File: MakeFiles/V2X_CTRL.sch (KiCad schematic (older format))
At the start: 22 parts, among them Q15 2N7000, U18 74HC595, U20 ATXMEGA128A4U-AU, X3 32.768K

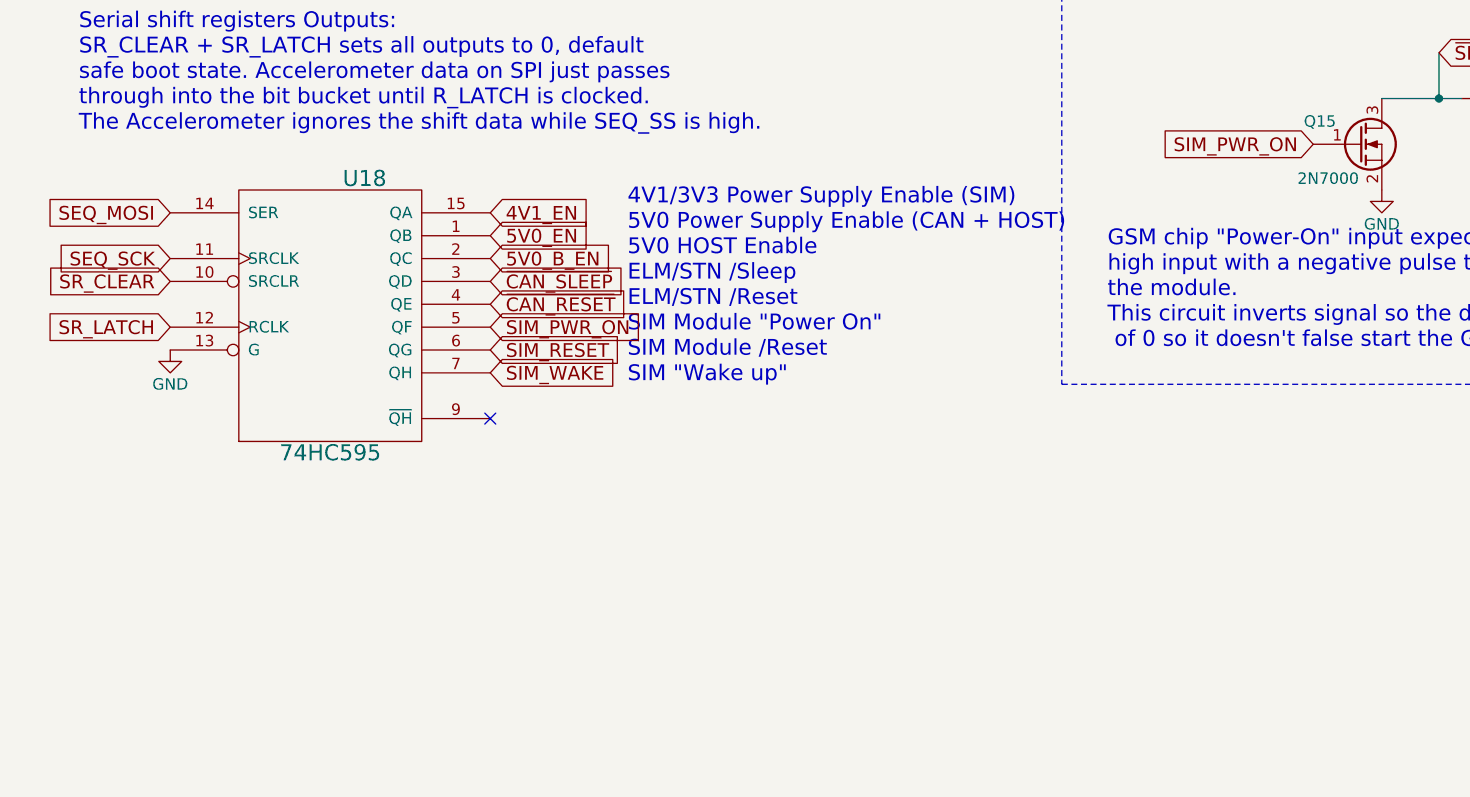
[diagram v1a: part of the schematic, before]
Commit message: Changes for documentation
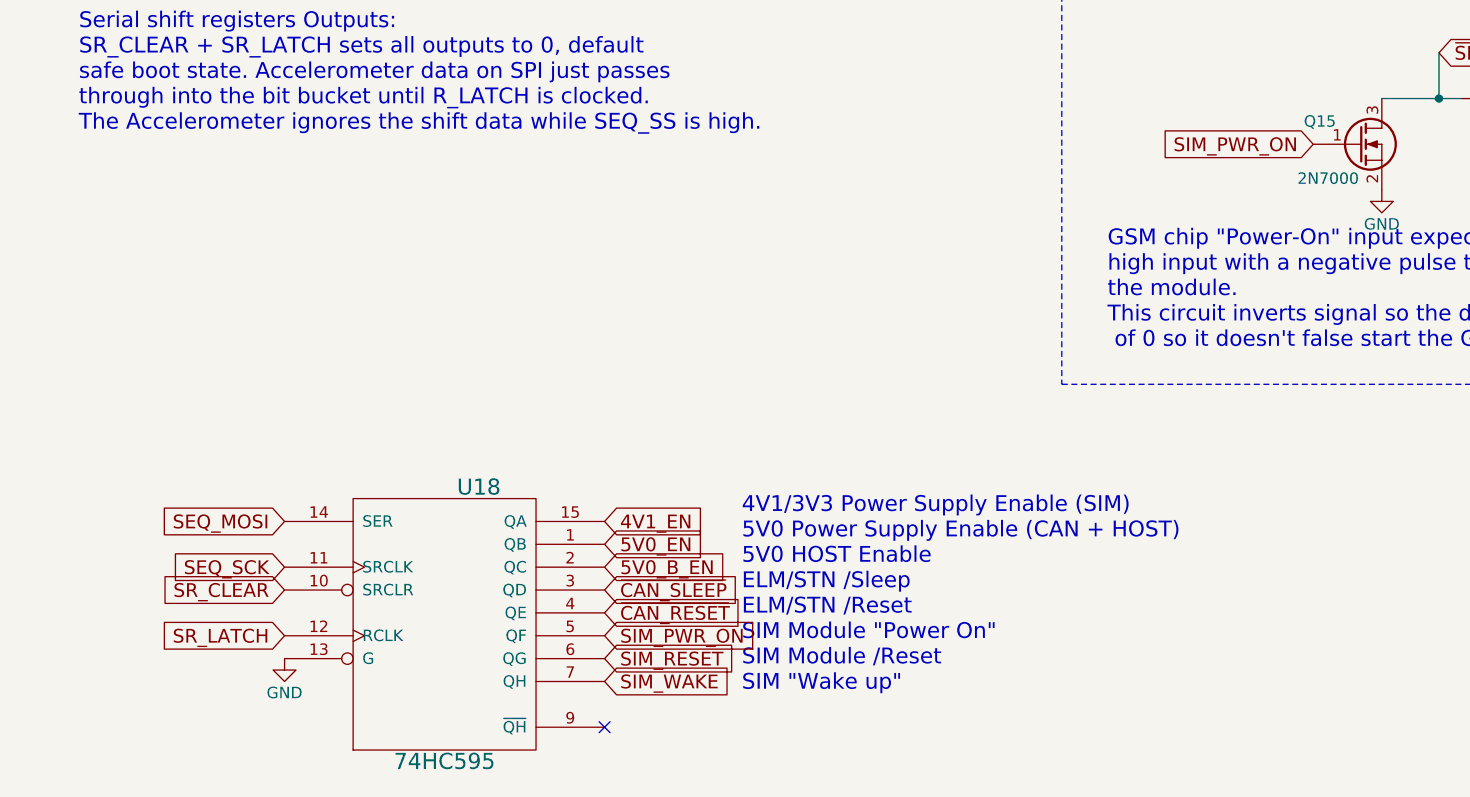
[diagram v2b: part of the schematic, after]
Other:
- moved on the sheet: U18
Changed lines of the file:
@@
 LIBS:xilinx
 LIBS:Zilog
+LIBS:CUSTOM_KICAD_PART
 LIBS:V2X-cache
 EELAYER 25 0
@@
 Text GLabel 6650 4450 2    60   Input ~ 0
 ~SIM_PWR_ON
-Text GLabel 2500 5750 2    60   Input ~ 0
+Text GLabel 3000 7100 2    60   Input ~ 0
 SIM_RESET
 Text GLabel 3350 3400 0    60   Input ~ 0
@@
 Text GLabel 3350 3200 0    60   Input ~ 0
 GPS_EN
-Text GLabel 2500 5150 2    60   Input ~ 0
+Text GLabel 3000 6500 2    60   Input ~ 0
 4V1_EN
-Text GLabel 2500 5250 2    60   Input ~ 0
+Text GLabel 3000 6600 2    60   Input ~ 0
 5V0_EN
 Text GLabel 3350 3000 0    60   Input ~ 0
 SIM_TXD
-Text GLabel 2500 5450 2    60   Input ~ 0
+Text GLabel 3000 6800 2    60   Input ~ 0
 ~CAN_SLEEP
-Text GLabel 2500 5550 2    60   Input ~ 0
+Text GLabel 3000 6900 2    60   Input ~ 0
 ~CAN_RESET
 Text Notes 6050 3600 0    69   ~ 0
@@
 Text Notes 8700 3000 0    60   ~ 0
 PDI (a-wire) Programing port
-Text Notes 3100 5900 0    69   ~ 0
+Text Notes 3600 7250 0    69   ~ 0
 4V1/3V3 Power Supply Enable (SIM)\n5V0 Power Supply Enable (CAN + HOST)\n5V0 HOST Enable \nELM/STN /Sleep\nELM/STN /Reset\nSIM Module "Power On"\nSIM Module /Reset\nSIM "Wake up"
 Text Notes 9700 3250 0    69   ~ 0
@@
 L 74HC595 U18
 U 1 1 55FA3B36
-P 1800 5600
-F 0 "U18" H 1950 6200 70  0000 C CNN
-F 1 "74HC595" H 1800 5000 70  0000 C CNN
-F 2 "Housings_SOIC:SOIC-16_3.9x9.9mm_Pitch1.27mm" H 1800 5600 60  0001 C CNN
-F 3 "http://www.mouser.com/ds/2/302/74HC_HCT595_Q100-269352.pdf" H 1800 5600 60  0001 C CNN
-F 4 "771-74HC595D-Q100" H 1800 5600 60  0001 C CNN "Mouse PN"
-	1    1800 5600
-	1    0    0    -1
-$EndComp
-Text GLabel 2500 5350 2    60   Input ~ 0
+P 2300 6950
+F 0 "U18" H 2450 7550 70  0000 C CNN
+F 1 "74HC595" H 2300 6350 70  0000 C CNN
+F 2 "Housings_SOIC:SOIC-16_3.9x9.9mm_Pitch1.27mm" H 2300 6950 60  0001 C CNN
+F 3 "http://www.mouser.com/ds/2/302/74HC_HCT595_Q100-269352.pdf" H 2300 6950 60  0001 C CNN
+F 4 "771-74HC595D-Q100" H 2300 6950 60  0001 C CNN "Mouse PN"
+	1    2300 6950
+	1    0    0    -1
+$EndComp
+Text GLabel 3000 6700 2    60   Input ~ 0
 5V0_B_EN
 $Comp
 L GND #PWR092
 U 1 1 55FA434A
-P 1100 5750
-F 0 "#PWR092" H 1100 5500 50  0001 C CNN
-F 1 "GND" H 1100 5600 50  0000 C CNN
-F 2 "" H 1100 5750 60  0000 C CNN
-F 3 "" H 1100 5750 60  0000 C CNN
-	1    1100 5750
+P 1600 7100
+F 0 "#PWR092" H 1600 6850 50  0001 C CNN
+F 1 "GND" H 1600 6950 50  0000 C CNN
+F 2 "" H 1600 7100 60  0000 C CNN
+F 3 "" H 1600 7100 60  0000 C CNN
+	1    1600 7100
 	1    0    0    -1
 $EndComp
@@
 Text GLabel 6100 4850 0    60   Input ~ 0
 SIM_PWR_ON
-Text GLabel 2500 5650 2    60   Input ~ 0
+Text GLabel 3000 7000 2    60   Input ~ 0
 SIM_PWR_ON
 Connection ~ 6650 4650
@@
 Text GLabel 7050 4650 2    60   Input ~ 0
 3V3
-Text GLabel 1100 5150 0    60   Input ~ 0
+Text GLabel 1600 6500 0    60   Input ~ 0
 SEQ_MOSI
-Text GLabel 1100 5650 0    60   Input ~ 0
+Text GLabel 1600 7000 0    60   Input ~ 0
 SR_LATCH
-Text GLabel 1100 5450 0    60   Input ~ 0
+Text GLabel 1600 6800 0    60   Input ~ 0
 SR_CLEAR
-Text GLabel 1100 5350 0    60   Input ~ 0
+Text GLabel 1600 6700 0    60   Input ~ 0
 SEQ_SCK
 Wire Notes Line
@@
 Text GLabel 5150 3100 2    60   Input ~ 0
 CAN_RXD
-Text GLabel 2500 5850 2    60   Input ~ 0
+Text GLabel 3000 7200 2    60   Input ~ 0
 SIM_WAKE
 NoConn ~ 9450 3550
@@
 Text GLabel 10650 4900 1    60   Input ~ 0
 4V1
-NoConn ~ 2500 6050
+NoConn ~ 3000 7400
 NoConn ~ 5150 2350
 NoConn ~ 5150 2550

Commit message: Part numer updates
for error or out of stock
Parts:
- C46: Mouse PN 603-CC603KRX7R7BB105 -> 81-GRM188R71C105KA2J
- U20: Mouse PN 556-ATXMEGA16A4U-AU -> 556-ATXMEGA128A4U-AU
- X3: Mouser 628-SC32P-125PF20PPM -> 815-S07AIG-32.76891T
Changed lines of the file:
@@
 SEQ_LED2
 $Comp
-L GND #PWR090
+L GND #PWR93
 U 1 1 55F86E9C
 P 4100 3900
-F 0 "#PWR090" H 4100 3650 50  0001 C CNN
+F 0 "#PWR93" H 4100 3650 50  0001 C CNN
 F 1 "GND" H 4100 3750 50  0000 C CNN
 F 2 "" H 4100 3900 60  0000 C CNN
@@
 PDI
 $Comp
-L GND #PWR091
+L GND #PWR102
 U 1 1 55F86EF0
 P 10000 3650
-F 0 "#PWR091" H 10000 3400 50  0001 C CNN
+F 0 "#PWR102" H 10000 3400 50  0001 C CNN
 F 1 "GND" H 10000 3500 50  0000 C CNN
 F 2 "" H 10000 3650 60  0000 C CNN
@@
 5V0_B_EN
 $Comp
-L GND #PWR092
+L GND #PWR90
 U 1 1 55FA434A
 P 1600 7100
-F 0 "#PWR092" H 1600 6850 50  0001 C CNN
+F 0 "#PWR90" H 1600 6850 50  0001 C CNN
 F 1 "GND" H 1600 6950 50  0000 C CNN
 F 2 "" H 1600 7100 60  0000 C CNN
@@
 $EndComp
 $Comp
-L GND #PWR093
+L GND #PWR94
 U 1 1 55FE1020
 P 6400 5050
-F 0 "#PWR093" H 6400 4800 50  0001 C CNN
+F 0 "#PWR94" H 6400 4800 50  0001 C CNN
 F 1 "GND" H 6400 4900 50  0000 C CNN
 F 2 "" H 6400 5050 60  0000 C CNN
@@
 Connection ~ 10550 750
 $Comp
-L GND #PWR094
+L GND #PWR103
 U 1 1 56006FBB
 P 10550 1100
-F 0 "#PWR094" H 10550 850 50  0001 C CNN
+F 0 "#PWR103" H 10550 850 50  0001 C CNN
 F 1 "GND" H 10550 950 50  0000 C CNN
 F 2 "" H 10550 1100 60  0000 C CNN
@@
 Connection ~ 9000 750
 $Comp
-L GND #PWR095
+L GND #PWR97
 U 1 1 560285A0
 P 9000 1100
-F 0 "#PWR095" H 9000 850 50  0001 C CNN
+F 0 "#PWR97" H 9000 850 50  0001 C CNN
 F 1 "GND" H 9000 950 50  0000 C CNN
 F 2 "" H 9000 1100 60  0000 C CNN
@@
 $EndComp
 $Comp
-L GND #PWR096
+L GND #PWR99
 U 1 1 560285F6
 P 9300 1100
-F 0 "#PWR096" H 9300 850 50  0001 C CNN
+F 0 "#PWR99" H 9300 850 50  0001 C CNN
 F 1 "GND" H 9300 950 50  0000 C CNN
 F 2 "" H 9300 1100 60  0000 C CNN
@@
 $EndComp
 $Comp
-L GND #PWR097
+L GND #PWR101
 U 1 1 5602864C
 P 9600 1100
-F 0 "#PWR097" H 9600 850 50  0001 C CNN
+F 0 "#PWR101" H 9600 850 50  0001 C CNN
 F 1 "GND" H 9600 950 50  0000 C CNN
 F 2 "" H 9600 1100 60  0000 C CNN
@@
 Connection ~ 9150 750
 $Comp
-L VCC #PWR098
+L VCC #PWR98
 U 1 1 56029609
 P 9150 700
-F 0 "#PWR098" H 9150 550 50  0001 C CNN
+F 0 "#PWR98" H 9150 550 50  0001 C CNN
 F 1 "VCC" H 9150 850 50  0000 C CNN
 F 2 "" H 9150 700 60  0000 C CNN
@@
 Connection ~ 8700 750
 $Comp
-L GND #PWR099
+L GND #PWR96
 U 1 1 5602C4DB
 P 8700 1100
-F 0 "#PWR099" H 8700 850 50  0001 C CNN
+F 0 "#PWR96" H 8700 850 50  0001 C CNN
 F 1 "GND" H 8700 950 50  0000 C CNN
 F 2 "" H 8700 1100 60  0000 C CNN
@@
 $EndComp
 $Comp
-L GND #PWR0100
+L GND #PWR95
 U 1 1 5602C537
 P 8400 1100
-F 0 "#PWR0100" H 8400 850 50  0001 C CNN
+F 0 "#PWR95" H 8400 850 50  0001 C CNN
 F 1 "GND" H 8400 950 50  0000 C CNN
 F 2 "" H 8400 1100 60  0000 C CNN
@@
 F 2 "CustomParts:C_0603_SM" H 10588 800 30  0001 C CNN
 F 3 "http://www.mouser.com/ds/2/447/UPY-GPHC_X7R_6.3V-to-50V_8-12304.pdf" H 10550 950 60  0001 C CNN
-F 4 "603-CC603KRX7R7BB105" H 10550 950 60  0001 C CNN "Mouse PN"
+F 4 "81-GRM188R71C105KA2J" H 10550 950 60  0001 C CNN "Mouse PN"
 	1    10550 950
 	1    0    0    -1
@@
 	9650 1800 9550 1800
 $Comp
-L GND #PWR0101
+L GND #PWR100
 U 1 1 56A15882
 P 9550 2100
-F 0 "#PWR0101" H 9550 1850 50  0001 C CNN
+F 0 "#PWR100" H 9550 1850 50  0001 C CNN
 F 1 "GND" H 9550 1950 50  0000 C CNN
 F 2 "" H 9550 2100 60  0000 C CNN
@@
 F 2 "Housings_QFP:TQFP-44_10x10mm_Pitch0.8mm" H 4250 2500 35  0001 C CIN
 F 3 "http://www.mouser.com/ds/2/36/Atmel-8387-8-and16-bit-AVR-Microcontroller-XMEGA-A-259135.pdf" H 4250 2500 60  0001 C CNN
-F 4 "556-ATXMEGA16A4U-AU" H 4250 2500 60  0001 C CNN "Mouse PN"
+F 4 "556-ATXMEGA128A4U-AU" H 4250 2500 60  0001 C CNN "Mouse PN"
 	1    4250 2500
 	1    0    0    -1
@@
 F 2 "Custom Parts:C_1206_SM" H 2150 2100 60  0001 C CNN
 F 3 "http://www.mouser.com/ds/2/360/SC-32P_Leaflet_r_newest-541780.pdf" H 2150 2100 60  0001 C CNN
-F 4 "628-SC32P-125PF20PPM" H 2150 2100 60  0001 C CNN "Mouser"
+F 4 "815-S07AIG-32.76891T" H 2150 2100 60  0001 C CNN "Mouser"
 	1    2150 2100
 	1    0    0    -1
@@
 	1850 2200 3350 2200
 $Comp
-L GND #PWR0102
+L GND #PWR92
 U 1 1 56DA1E3F
 P 2450 1800
-F 0 "#PWR0102" H 2450 1550 50  0001 C CNN
+F 0 "#PWR92" H 2450 1550 50  0001 C CNN
 F 1 "GND" H 2450 1650 50  0000 C CNN
 F 2 "" H 2450 1800 60  0000 C CNN
@@
 $EndComp
 $Comp
-L GND #PWR0103
+L GND #PWR91
 U 1 1 56DA2162
 P 1850 1800
-F 0 "#PWR0103" H 1850 1550 50  0001 C CNN
+F 0 "#PWR91" H 1850 1550 50  0001 C CNN
 F 1 "GND" H 1850 1650 50  0000 C CNN
 F 2 "" H 1850 1800 60  0000 C CNN

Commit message: Rev2.1 produced
Built R2.0, included findings, minor tweaks to placment and BOM.
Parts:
- C46: Mouse PN 81-GRM188R71C105KA2J -> 581-06036C105MAT2A
- C53, C54: Mouse PN 810-C1608C0G1H090C -> 81-GRM1885C1H9R0DA1D; Mouser DNS -> (none)
- R63: Mouse PN 71-CRCW0603-220-E3 -> 667-ERJ-3GEYJ221V
- X3: Mouse PN (none) -> 815-S07AIG-32.76891T; Mouser 815-S07AIG-32.76891T -> (none)
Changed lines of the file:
@@
 SEQ_LED2
 $Comp
-L GND #PWR93
+L GND #PWR090
 U 1 1 55F86E9C
 P 4100 3900
-F 0 "#PWR93" H 4100 3650 50  0001 C CNN
+F 0 "#PWR090" H 4100 3650 50  0001 C CNN
 F 1 "GND" H 4100 3750 50  0000 C CNN
 F 2 "" H 4100 3900 60  0000 C CNN
@@
 PDI
 $Comp
-L GND #PWR102
+L GND #PWR091
 U 1 1 55F86EF0
 P 10000 3650
-F 0 "#PWR102" H 10000 3400 50  0001 C CNN
+F 0 "#PWR091" H 10000 3400 50  0001 C CNN
 F 1 "GND" H 10000 3500 50  0000 C CNN
 F 2 "" H 10000 3650 60  0000 C CNN
@@
 5V0_B_EN
 $Comp
-L GND #PWR90
+L GND #PWR092
 U 1 1 55FA434A
 P 1600 7100
-F 0 "#PWR90" H 1600 6850 50  0001 C CNN
+F 0 "#PWR092" H 1600 6850 50  0001 C CNN
 F 1 "GND" H 1600 6950 50  0000 C CNN
 F 2 "" H 1600 7100 60  0000 C CNN
@@
 $EndComp
 $Comp
-L GND #PWR94
+L GND #PWR093
 U 1 1 55FE1020
 P 6400 5050
-F 0 "#PWR94" H 6400 4800 50  0001 C CNN
+F 0 "#PWR093" H 6400 4800 50  0001 C CNN
 F 1 "GND" H 6400 4900 50  0000 C CNN
 F 2 "" H 6400 5050 60  0000 C CNN
@@
 Connection ~ 10550 750
 $Comp
-L GND #PWR103
+L GND #PWR094
 U 1 1 56006FBB
 P 10550 1100
-F 0 "#PWR103" H 10550 850 50  0001 C CNN
+F 0 "#PWR094" H 10550 850 50  0001 C CNN
 F 1 "GND" H 10550 950 50  0000 C CNN
 F 2 "" H 10550 1100 60  0000 C CNN
@@
 Connection ~ 9000 750
 $Comp
-L GND #PWR97
+L GND #PWR095
 U 1 1 560285A0
 P 9000 1100
-F 0 "#PWR97" H 9000 850 50  0001 C CNN
+F 0 "#PWR095" H 9000 850 50  0001 C CNN
 F 1 "GND" H 9000 950 50  0000 C CNN
 F 2 "" H 9000 1100 60  0000 C CNN
@@
 $EndComp
 $Comp
-L GND #PWR99
+L GND #PWR096
 U 1 1 560285F6
 P 9300 1100
-F 0 "#PWR99" H 9300 850 50  0001 C CNN
+F 0 "#PWR096" H 9300 850 50  0001 C CNN
 F 1 "GND" H 9300 950 50  0000 C CNN
 F 2 "" H 9300 1100 60  0000 C CNN
@@
 $EndComp
 $Comp
-L GND #PWR101
+L GND #PWR097
 U 1 1 5602864C
 P 9600 1100
-F 0 "#PWR101" H 9600 850 50  0001 C CNN
+F 0 "#PWR097" H 9600 850 50  0001 C CNN
 F 1 "GND" H 9600 950 50  0000 C CNN
 F 2 "" H 9600 1100 60  0000 C CNN
@@
 Connection ~ 9150 750
 $Comp
-L VCC #PWR98
+L VCC #PWR098
 U 1 1 56029609
 P 9150 700
-F 0 "#PWR98" H 9150 550 50  0001 C CNN
+F 0 "#PWR098" H 9150 550 50  0001 C CNN
 F 1 "VCC" H 9150 850 50  0000 C CNN
 F 2 "" H 9150 700 60  0000 C CNN
@@
 Connection ~ 8700 750
 $Comp
-L GND #PWR96
+L GND #PWR099
 U 1 1 5602C4DB
 P 8700 1100
-F 0 "#PWR96" H 8700 850 50  0001 C CNN
+F 0 "#PWR099" H 8700 850 50  0001 C CNN
 F 1 "GND" H 8700 950 50  0000 C CNN
 F 2 "" H 8700 1100 60  0000 C CNN
@@
 $EndComp
 $Comp
-L GND #PWR95
+L GND #PWR0100
 U 1 1 5602C537
 P 8400 1100
-F 0 "#PWR95" H 8400 850 50  0001 C CNN
+F 0 "#PWR0100" H 8400 850 50  0001 C CNN
 F 1 "GND" H 8400 950 50  0000 C CNN
 F 2 "" H 8400 1100 60  0000 C CNN
@@
 F 2 "CustomParts:C_0603_SM" H 10588 800 30  0001 C CNN
 F 3 "http://www.mouser.com/ds/2/447/UPY-GPHC_X7R_6.3V-to-50V_8-12304.pdf" H 10550 950 60  0001 C CNN
-F 4 "81-GRM188R71C105KA2J" H 10550 950 60  0001 C CNN "Mouse PN"
+F 4 "581-06036C105MAT2A" H 10550 950 60  0001 C CNN "Mouse PN"
 	1    10550 950
 	1    0    0    -1
@@
 F 2 "CustomParts:R_0603_sm" V 9730 5050 30  0001 C CNN
 F 3 "http://www.mouser.com/ds/2/427/dcrcwe3-109170.pdf" H 9800 5050 30  0001 C CNN
-F 4 "71-CRCW0603-220-E3" H 9800 5050 60  0001 C CNN "Mouse PN"
+F 4 "667-ERJ-3GEYJ221V" H 9800 5050 60  0001 C CNN "Mouse PN"
 	1    9800 5050
 	-1   0    0    1
@@
 	9650 1800 9550 1800
 $Comp
-L GND #PWR100
+L GND #PWR0101
 U 1 1 56A15882
 P 9550 2100
-F 0 "#PWR100" H 9550 1850 50  0001 C CNN
+F 0 "#PWR0101" H 9550 1850 50  0001 C CNN
 F 1 "GND" H 9550 1950 50  0000 C CNN
 F 2 "" H 9550 2100 60  0000 C CNN
@@
 F 2 "Custom Parts:C_1206_SM" H 2150 2100 60  0001 C CNN
 F 3 "http://www.mouser.com/ds/2/360/SC-32P_Leaflet_r_newest-541780.pdf" H 2150 2100 60  0001 C CNN
-F 4 "815-S07AIG-32.76891T" H 2150 2100 60  0001 C CNN "Mouser"
+F 4 "815-S07AIG-32.76891T" H 2150 2100 60  0001 C CNN "Mouse PN"
 	1    2150 2100
 	1    0    0    -1
@@
 F 1 "9p" H 1875 1850 50  0000 L CNN
 F 2 "CustomParts:C_0603_SM" H 1888 1800 30  0001 C CNN
-F 3 "http://www.mouser.com/ds/2/400/lcc_commercial_general_en-837201.pdf" H 1850 1950 60  0001 C CNN
-F 4 "DNS" H 1850 1950 60  0001 C CNN "Mouser"
-F 5 "810-C1608C0G1H090C" H 1850 1950 60  0001 C CNN "Mouse PN"
+F 3 "http://www.mouser.com/ds/2/281/c02e-2905.pdf" H 1850 1950 60  0001 C CNN
+F 4 "81-GRM1885C1H9R0DA1D" H 1850 1950 60  0001 C CNN "Mouse PN"
 	1    1850 1950
 	-1   0    0    -1
@@
 F 1 "9p" H 2475 1850 50  0000 L CNN
 F 2 "CustomParts:C_0603_SM" H 2488 1800 30  0001 C CNN
-F 3 "http://www.mouser.com/ds/2/400/lcc_commercial_general_en-837201.pdf" H 2450 1950 60  0001 C CNN
-F 4 "DNS" H 2450 1950 60  0001 C CNN "Mouser"
-F 5 "810-C1608C0G1H090C" H 2450 1950 60  0001 C CNN "Mouse PN"
+F 3 "http://www.mouser.com/ds/2/281/c02e-2905.pdf" H 2450 1950 60  0001 C CNN
+F 4 "81-GRM1885C1H9R0DA1D" H 2450 1950 60  0001 C CNN "Mouse PN"
 	1    2450 1950
 	-1   0    0    -1
@@
 	1850 2200 3350 2200
 $Comp
-L GND #PWR92
+L GND #PWR0102
 U 1 1 56DA1E3F
 P 2450 1800
-F 0 "#PWR92" H 2450 1550 50  0001 C CNN
+F 0 "#PWR0102" H 2450 1550 50  0001 C CNN
 F 1 "GND" H 2450 1650 50  0000 C CNN
 F 2 "" H 2450 1800 60  0000 C CNN
@@
 $EndComp
 $Comp
-L GND #PWR91
+L GND #PWR0103
 U 1 1 56DA2162
 P 1850 1800
-F 0 "#PWR91" H 1850 1550 50  0001 C CNN
+F 0 "#PWR0103" H 1850 1550 50  0001 C CNN
 F 1 "GND" H 1850 1650 50  0000 C CNN
 F 2 "" H 1850 1800 60  0000 C CNN
